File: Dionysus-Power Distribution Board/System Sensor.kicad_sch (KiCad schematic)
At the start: 19 parts

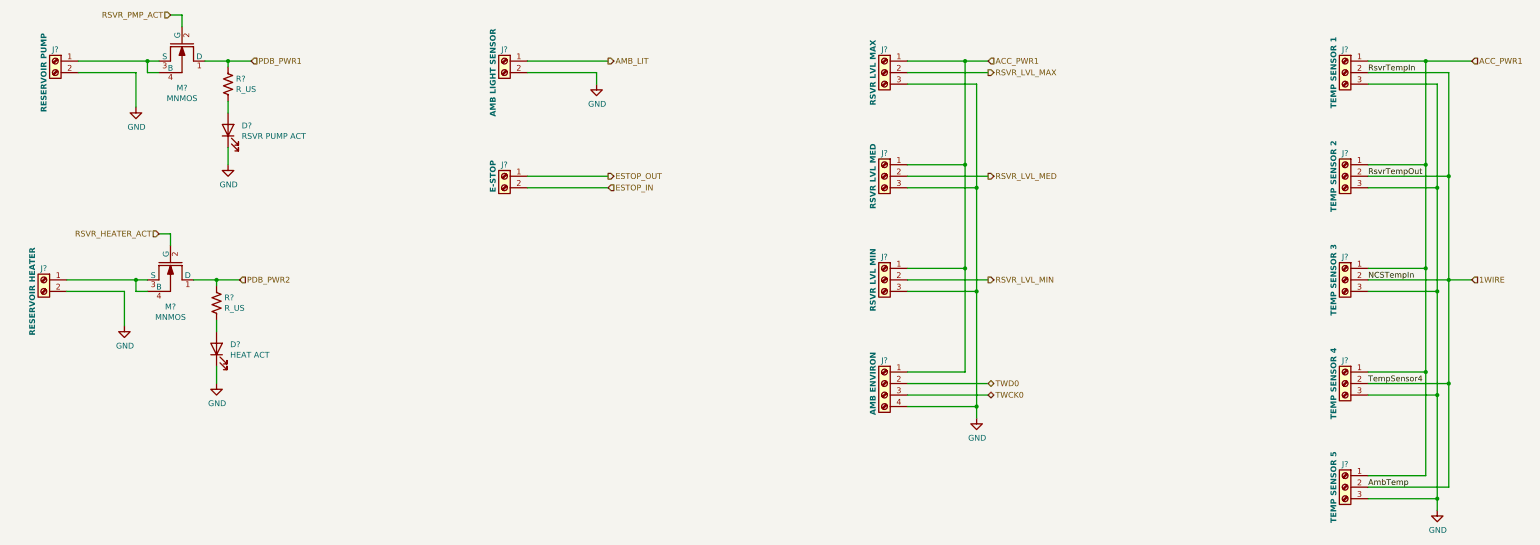
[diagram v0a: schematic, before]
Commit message: Added Libraries and Copied previous work
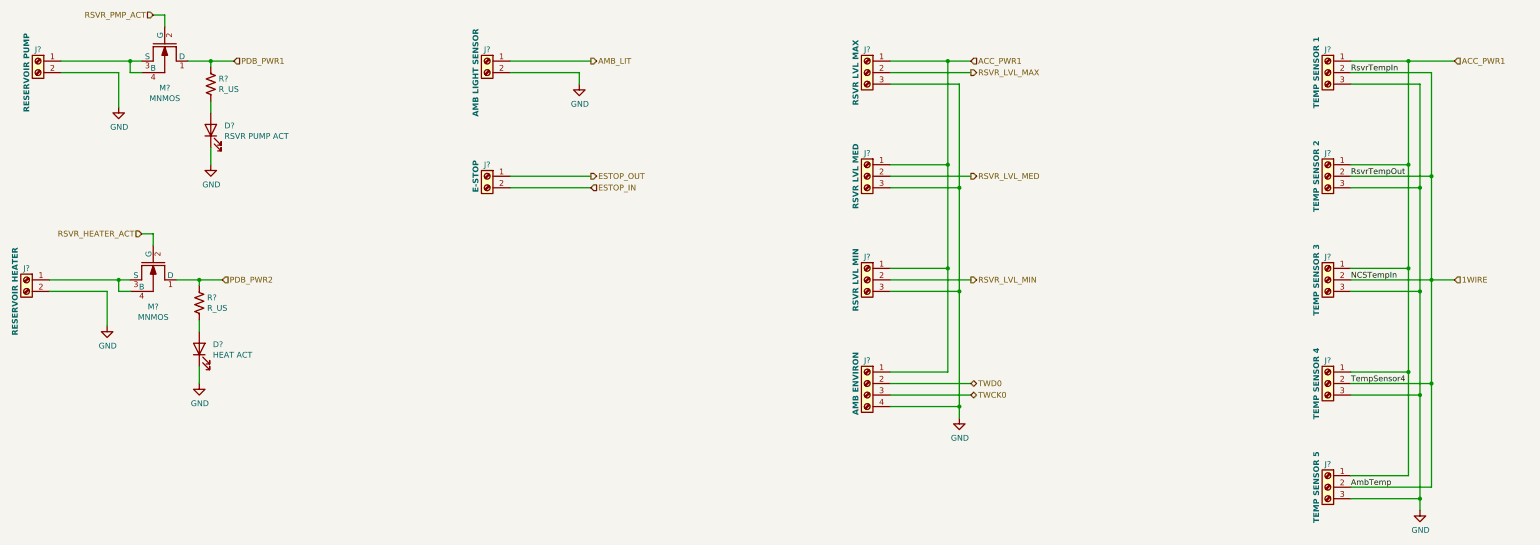
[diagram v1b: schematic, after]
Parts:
- removed D?: HEAT ACT, symbol Device:LED
- removed D?: RSVR PUMP ACT, symbol Device:LED
- removed J?: AMB ENVIRON, symbol Connector:Screw_Terminal_01x04
- removed J?: RSVR LVL MIN, TerminalBlock_Phoenix:TerminalBlock_Phoenix_MKDS-1,5-3_1x03_P5.00mm_Horizontal, symbol Connector:Screw_Terminal_01x03
- removed J?: RESERVOIR PUMP, symbol Connector:Screw_Terminal_01x02
- removed J?: TEMP SENSOR 2, TerminalBlock_Phoenix:TerminalBlock_Phoenix_MKDS-1,5-3_1x03_P5.00mm_Horizontal, symbol Connector:Screw_Terminal_01x03
- removed J?: TEMP SENSOR 5, TerminalBlock_Phoenix:TerminalBlock_Phoenix_MKDS-1,5-3_1x03_P5.00mm_Horizontal, symbol Connector:Screw_Terminal_01x03
- removed J?: TEMP SENSOR 1, TerminalBlock_Phoenix:TerminalBlock_Phoenix_MKDS-1,5-3_1x03_P5.00mm_Horizontal, symbol Connector:Screw_Terminal_01x03
- removed J?: RESERVOIR HEATER, symbol Connector:Screw_Terminal_01x02
- removed J?: RSVR LVL MAX, TerminalBlock_Phoenix:TerminalBlock_Phoenix_MKDS-1,5-3_1x03_P5.00mm_Horizontal, symbol Connector:Screw_Terminal_01x03
- removed J?: E-STOP, symbol Connector:Screw_Terminal_01x02
- removed J?: RSVR LVL MED, TerminalBlock_Phoenix:TerminalBlock_Phoenix_MKDS-1,5-3_1x03_P5.00mm_Horizontal, symbol Connector:Screw_Terminal_01x03
- removed J?: TEMP SENSOR 4, TerminalBlock_Phoenix:TerminalBlock_Phoenix_MKDS-1,5-3_1x03_P5.00mm_Horizontal, symbol Connector:Screw_Terminal_01x03
- removed J?: AMB LIGHT SENSOR, symbol Connector:Screw_Terminal_01x02
- removed J?: TEMP SENSOR 3, TerminalBlock_Phoenix:TerminalBlock_Phoenix_MKDS-1,5-3_1x03_P5.00mm_Horizontal, symbol Connector:Screw_Terminal_01x03
- removed M? (x2): MNMOS, symbol Power Distribution Board-rescue:MNMOS-pspice
- removed R? (x2): R_US, symbol Device:R_US
- added D?: RSVR PUMP ACT, symbol Device:LED
- added D?: HEAT ACT, symbol Device:LED
- added J?: TEMP SENSOR 2, TerminalBlock_Phoenix:TerminalBlock_Phoenix_MKDS-1,5-3_1x03_P5.00mm_Horizontal, symbol Connector:Screw_Terminal_01x03
- added J?: RESERVOIR HEATER, symbol Connector:Screw_Terminal_01x02
- added J?: RSVR LVL MED, TerminalBlock_Phoenix:TerminalBlock_Phoenix_MKDS-1,5-3_1x03_P5.00mm_Horizontal, symbol Connector:Screw_Terminal_01x03
- added J?: TEMP SENSOR 5, TerminalBlock_Phoenix:TerminalBlock_Phoenix_MKDS-1,5-3_1x03_P5.00mm_Horizontal, symbol Connector:Screw_Terminal_01x03
- added J?: TEMP SENSOR 4, TerminalBlock_Phoenix:TerminalBlock_Phoenix_MKDS-1,5-3_1x03_P5.00mm_Horizontal, symbol Connector:Screw_Terminal_01x03
- added J?: TEMP SENSOR 1, TerminalBlock_Phoenix:TerminalBlock_Phoenix_MKDS-1,5-3_1x03_P5.00mm_Horizontal, symbol Connector:Screw_Terminal_01x03
- added J?: RESERVOIR PUMP, symbol Connector:Screw_Terminal_01x02
- added J?: AMB LIGHT SENSOR, symbol Connector:Screw_Terminal_01x02
- added J?: RSVR LVL MAX, TerminalBlock_Phoenix:TerminalBlock_Phoenix_MKDS-1,5-3_1x03_P5.00mm_Horizontal, symbol Connector:Screw_Terminal_01x03
- added J?: E-STOP, symbol Connector:Screw_Terminal_01x02
- added J?: AMB ENVIRON, symbol Connector:Screw_Terminal_01x04
- added J?: TEMP SENSOR 3, TerminalBlock_Phoenix:TerminalBlock_Phoenix_MKDS-1,5-3_1x03_P5.00mm_Horizontal, symbol Connector:Screw_Terminal_01x03
- added J?: RSVR LVL MIN, TerminalBlock_Phoenix:TerminalBlock_Phoenix_MKDS-1,5-3_1x03_P5.00mm_Horizontal, symbol Connector:Screw_Terminal_01x03
- added M? (x2): MNMOS, symbol Power Distribution Board-rescue:MNMOS-pspice
- added R? (x2): R_US, symbol Device:R_US
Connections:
- net 1WIRE: now also J?.2 (Pin_2), J?.2 (Pin_2), J?.2 (Pin_2), J?.2 (Pin_2), J?.2 (Pin_2)
- net ACC_PWR1: now also J?.1 (Pin_1), J?.1 (Pin_1), J?.1 (Pin_1), J?.1 (Pin_1), J?.1 (Pin_1), J?.1 (Pin_1), J?.1 (Pin_1), J?.1 (Pin_1), J?.1 (Pin_1)
- net AMB_LIT: now also J?.1 (Pin_1)
- net ESTOP_IN: now also J?.2 (Pin_2)
- net ESTOP_OUT: now also J?.1 (Pin_1)
- net GND: now also D?.1 (K), D?.1 (K), J?.2 (Pin_2), J?.2 (Pin_2), J?.2 (Pin_2), J?.3 (Pin_3), J?.3 (Pin_3), J?.3 (Pin_3), J?.3 (Pin_3), J?.3 (Pin_3), J?.3 (Pin_3), J?.3 (Pin_3), J?.3 (Pin_3), J?.4 (Pin_4)
- net PDB_PWR1: now also M?.1 (D), R?.1
- net PDB_PWR2: now also M?.1 (D), R?.1
- net RSVR_HEATER_ACT: now also M?.2 (G)
- net RSVR_LVL_MAX: now also J?.2 (Pin_2)
- net RSVR_LVL_MED: now also J?.2 (Pin_2)
- net RSVR_LVL_MIN: now also J?.2 (Pin_2)
- net RSVR_PMP_ACT: now also M?.2 (G)
- net TWCK0: now also J?.3 (Pin_3)
- net TWD0: now also J?.2 (Pin_2)
- new net: D?.2 (A), R?.2 (x2)
- new net: J?.1 (Pin_1), M?.3 (S), M?.4 (B) (x2)
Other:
- title: Power Distribution Board, Dionysus -> (none)
